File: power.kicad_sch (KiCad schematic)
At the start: 13 parts, among them U1 B0505S-1WR2, U22 TLV76733DRVx

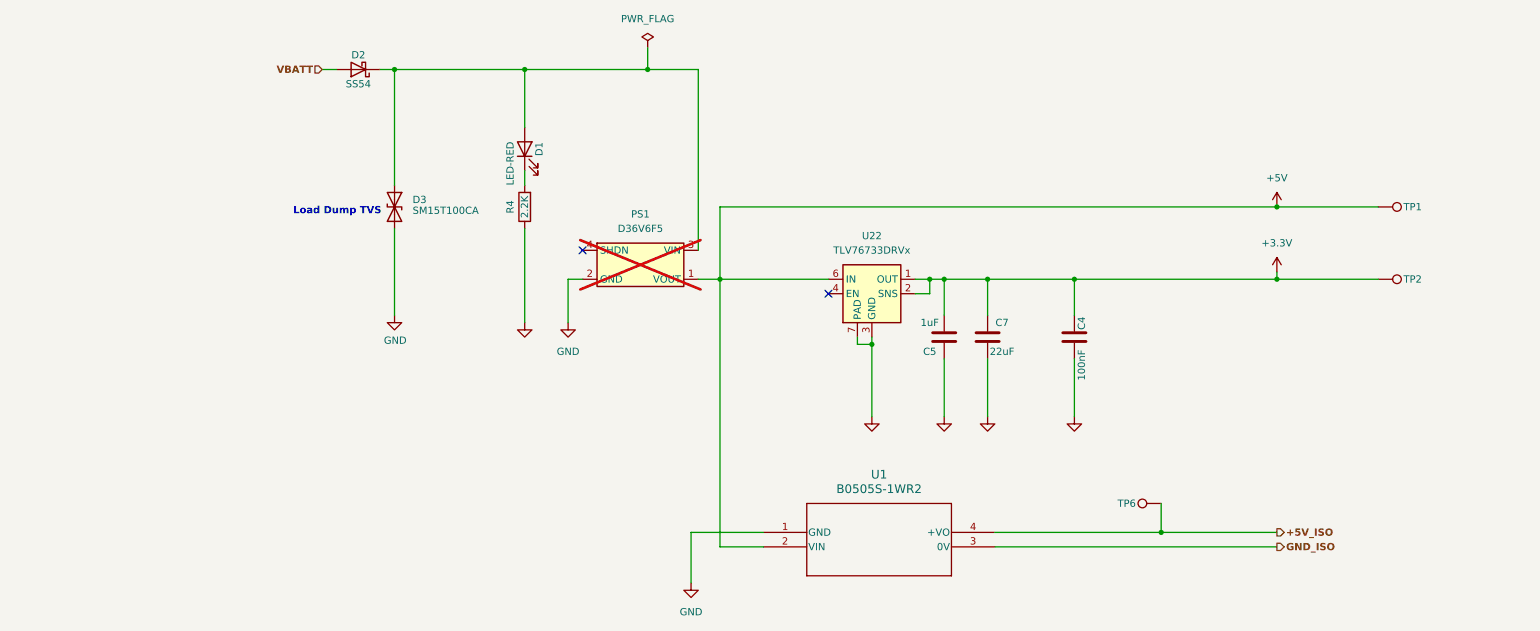
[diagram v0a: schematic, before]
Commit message: version 2 changes
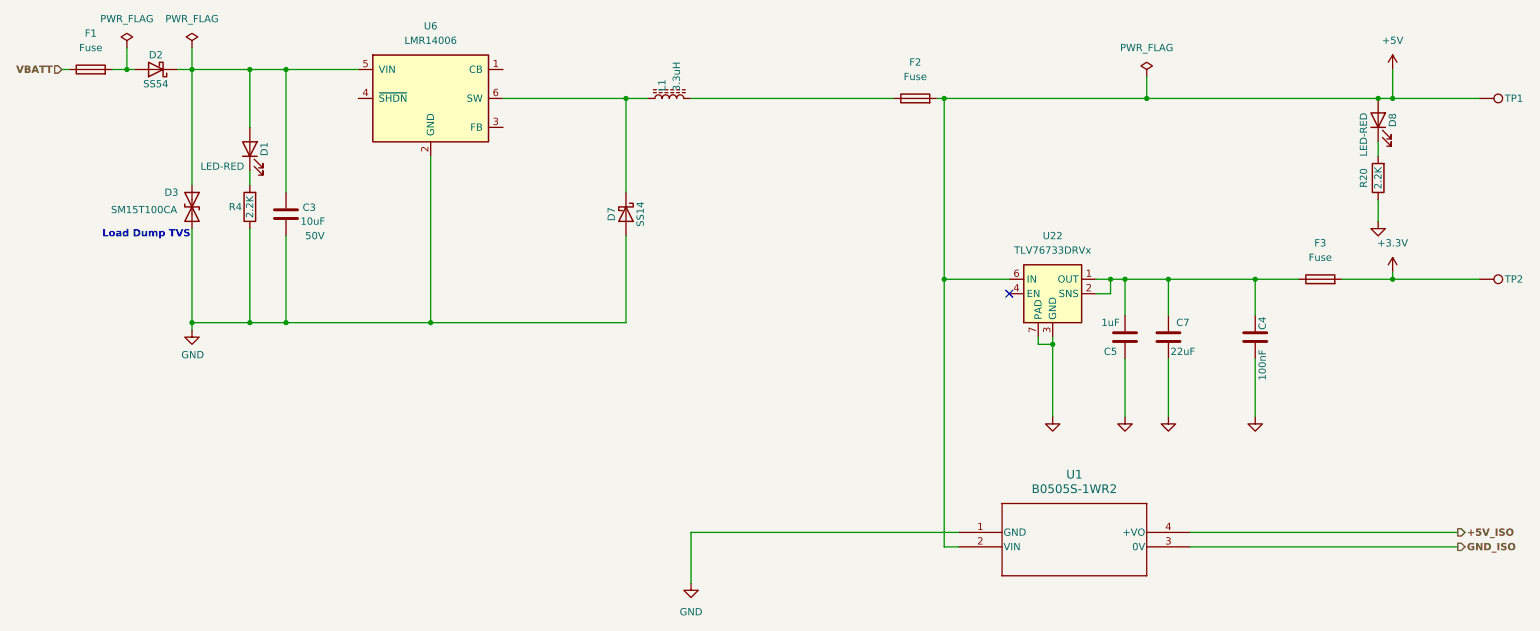
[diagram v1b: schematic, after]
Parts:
- removed PS1: D36V6F5, Connector_PinHeader_2.54mm:PinHeader_1x04_P2.54mm_Vertical, symbol dnt:D36V6F5
- removed TP6: 5V ISO, dnt:TestPoint_Pad_D1.0mm FP .6R, symbol Connector:TestPoint
- added C3: 10uF, Capacitor_SMD:C_0805_2012Metric, symbol Device:C
- added D7: SS14, dnt:D_SMA - polarity, symbol Diode:B340
- added D8: LED-RED, LED_SMD:LED_0603_1608Metric, symbol Device:LED
- added F1, F2, F3: Fuse, Fuse:Fuse_0805_2012Metric, symbol Device:Fuse
- added L1: 3.3uH, Inductor_SMD:L_Sunlord_SWPA4030S, symbol Device:L_Ferrite
- added R20: 2.2K, Resistor_SMD:R_0603_1608Metric, symbol Device:R
- added U6: LMR14006, Package_TO_SOT_SMD:SOT-23-6, symbol Regulator_Switching:LMR14206
- D2: footprint Diode_SMD:D_SMA -> dnt:D_SMA - polarity
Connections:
- net +3.3V: now also F3.2; no longer C4.1, C5.2, C7.1, U22.1 (OUT), U22.2 (SNS)
- net +5V: now also D8.2 (A), F2.2
- net GND: now also C3.2, D7.2 (A), R20.1, U6.2 (GND)
- net VBATT: now also F1.1; no longer D2.2 (A)
- net at D1.2 (A), D2.1 (K), D3.1 (A1): now also C3.1, U6.5 (VIN)
- new net: C4.1, C5.2, C7.1, F3.1, U22.1 (OUT), U22.2 (SNS)
- new net: D2.2 (A), F1.2
- new net: D7.1 (K), L1.1, U6.6 (SW)
- new net: F2.1, L1.2
- new net: D8.1 (K), R20.2
- no-connect marks 2 -> 1
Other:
- moved on the sheet: C4, C5, C7, D1, D2, D3, R4, TP1, TP2, U1, U22
